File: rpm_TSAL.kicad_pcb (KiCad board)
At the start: 4 copper layers, 123 parts, among them J1 Conn_01x02, J14 Conn_01x04, J2 Conn_01x04, J3 Conn_01x04, J4 Conn_01x04, J6 Conn_01x02, J7 Conn_01x02, Q1 NMOS, Q2 NMOS, Q3 NMOS, Q4 NMOS, Q5 PMOS, Q7 NMOS, U1 OPA355NA, U10 SN74HCS266PWR, U11 OPA355NA, U12 74LVC1G32GV, U13 SFH617A-1X007T, U14 OPA355NA, U15 TBA1-1211E, U16 TBA1-0511E, U17 TBA1-0511E, U18 IP4252CZ16, U2 L7805, U3 74LVC2G74, U4 SFH617A-1X007T, U5 NE555D, U6 CD74HC30PWR, U7 4072, U8 4001, U9 74LVC1G32GV

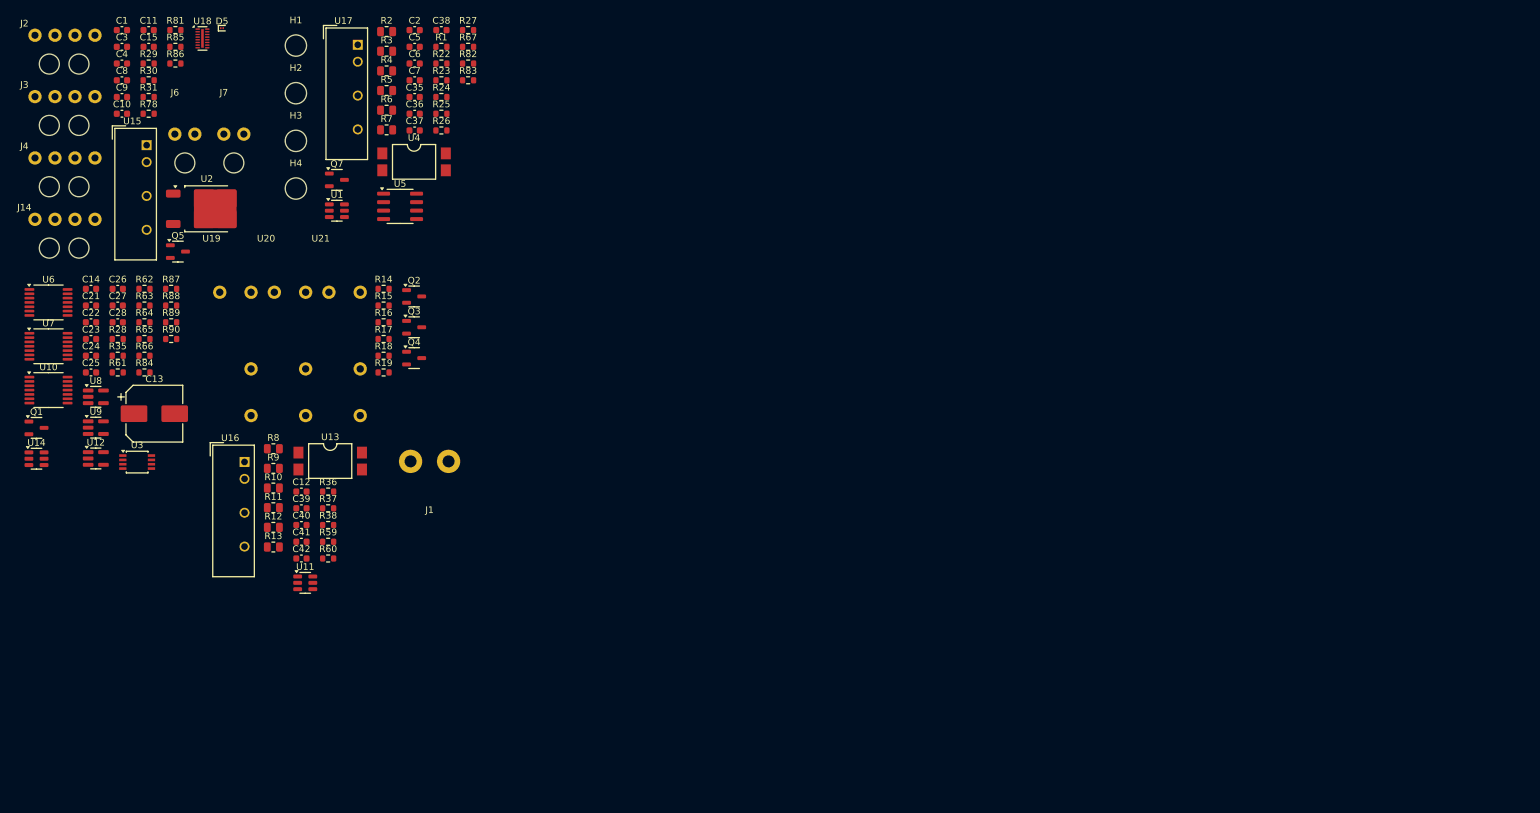
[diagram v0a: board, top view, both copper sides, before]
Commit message: Added Sub project
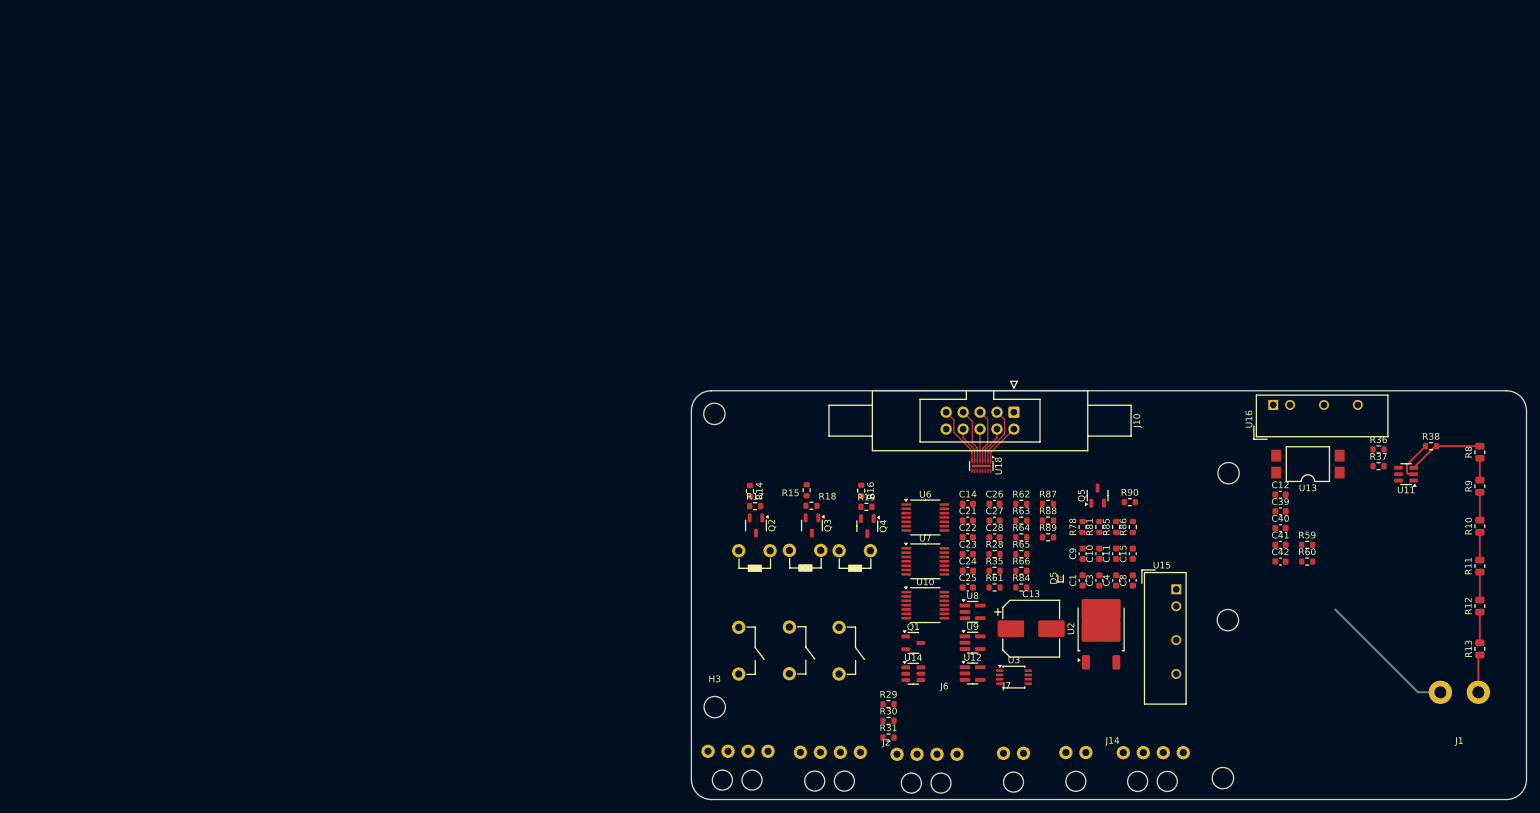
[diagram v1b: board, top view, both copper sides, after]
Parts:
- removed C2, C36, C38, C5, C6, C7: 100nF, Capacitor_SMD:C_0603_1608Metric
- removed C35, C37: 10uF, Capacitor_SMD:C_0603_1608Metric
- removed Q7: NMOS, Package_TO_SOT_SMD:SOT-23-3
- removed R1, R22, R23, R25, R26, R67: 1k, Resistor_SMD:R_0603_1608Metric
- removed R2, R3, R4, R5, R6, R7: 52k3, Resistor_SMD:R_0805_2012Metric
- removed R24: 12k, Resistor_SMD:R_0603_1608Metric
- removed R27, R83: 10k, Resistor_SMD:R_0603_1608Metric
- removed R82: 200R, Resistor_SMD:R_0603_1608Metric
- removed U1: OPA355NA, Package_TO_SOT_SMD:SOT-23-6
- removed U17: TBA1-0511E, Converter_DCDC:Converter_DCDC_TRACO_TBA1-xxxxE_Single_THT
- removed U4: SFH617A-1X007T, Package_DIP:SMDIP-4_W9.53mm_Clearance8mm
- removed U5: NE555D, Package_SO:SOIC-8_3.9x4.9mm_P1.27mm
- added H5: MountingHole, MountingHole:MountingHole_3.2mm_M3, F.Cu at (129.1, 76.5)
- added J10: Conn_01x10, Connector_IDC:IDC-Header_2x05_P2.54mm_Latch6.5mm_Vertical, F.Cu at (174.0, 76.2)
- H1, H2, H3, H4: footprint MountingHole:MountingHole_3.2mm_M3_DIN965 -> MountingHole:MountingHole_3.2mm_M3
- U19, U20, U21: moved to B.Cu
- moved J14 181.8 mm to (188.8, 126.0)
- moved R13 181.7 mm to (243.9, 111.7), turned to 90 degrees
- moved R12 181.4 mm to (243.9, 105.3), turned to -90 degrees
- moved R11 181.2 mm to (243.9, 99.3), turned to -90 degrees
- moved R10 181.1 mm to (243.9, 93.3), turned to 90 degrees
- moved R9 181.0 mm to (243.9, 87.3), turned to 90 degrees
- moved R8 181.0 mm to (243.9, 82.2), turned to 90 degrees
- moved C8 169.2 mm to (191.8, 101.4), turned to 90 degrees
- moved J2 168.4 mm to (154.9, 126.2)
- moved U15 168.2 mm to (198.3, 102.8)
- moved C4 168.1 mm to (189.3, 101.4), turned to 90 degrees
- moved C3 167.1 mm to (186.8, 101.4), turned to 90 degrees
- moved C1 166.1 mm to (184.3, 101.4), turned to 90 degrees
- moved C15 166.1 mm to (191.8, 97.4), turned to 90 degrees
- moved U11 166.0 mm to (232.8, 85.5), turned to 180 degrees
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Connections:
- J1 pad 1: HV+ -> HV-
- J1 pad 2: HV- -> HV+
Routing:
- net HV-: track 0.00 -> 27.2 mm
- net Net-(U11-+): track 0.00 -> 11.1 mm
- net Net-(J10-Pin_9): track 0.00 -> 8.90 mm
- net Net-(J10-Pin_3): track 0.00 -> 8.86 mm
- net Net-(J10-Pin_7): track 0.00 -> 8.23 mm
- net Net-(J10-Pin_5): track 0.00 -> 8.14 mm
- net Net-(J10-Pin_2): track 0.00 -> 6.26 mm
- net HV+: track 0.00 -> 5.70 mm
- net Net-(J10-Pin_4): track 0.00 -> 5.53 mm
- net Net-(J10-Pin_8): track 0.00 -> 5.53 mm
- net Net-(J10-Pin_6): track 0.00 -> 4.81 mm
- net Net-(R12-Pad2): track 0.00 -> 4.60 mm
- net Net-(R10-Pad2): track 0.00 -> 4.18 mm
- net Net-(R11-Pad2): track 0.00 -> 4.17 mm
- net Net-(R10-Pad1): track 0.00 -> 4.15 mm
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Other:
- board outline added: 125.3 x 61.3 mm
- board text added: "Isolating Case over LV Section"
